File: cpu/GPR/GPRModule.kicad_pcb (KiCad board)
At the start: 2 copper layers, 100 x 80 mm, 52 parts, among them J1 Interconnect, U1 74HCT574, U10 74LHCT45, U11 74HCT125, U2 74HCT574, U3 74HCT245, U4 74HCT245, U5 74HCT245, U6 74HCT245, U7 74HCT245, U8 74HCT245, U9 74HCT245

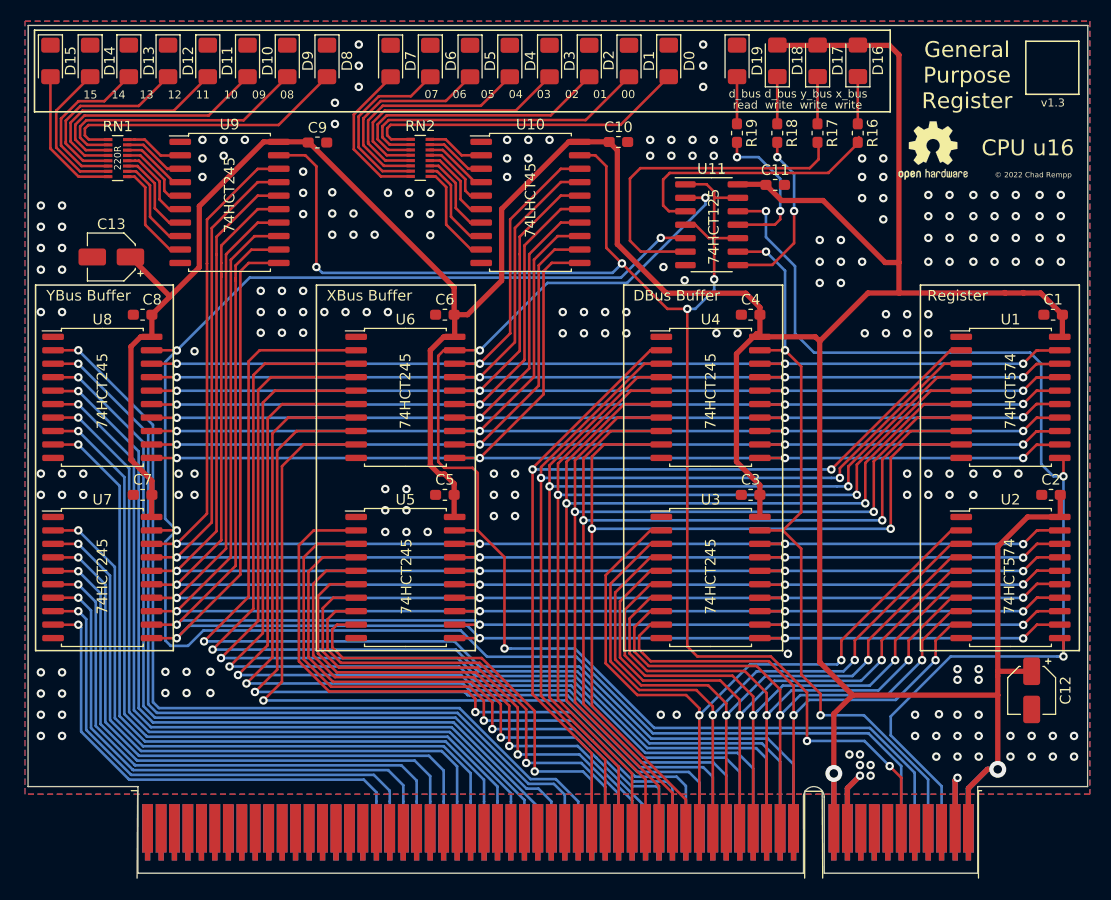
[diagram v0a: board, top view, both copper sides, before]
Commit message: Upgrade to KiCad 6 and commit a bunch of random stuff
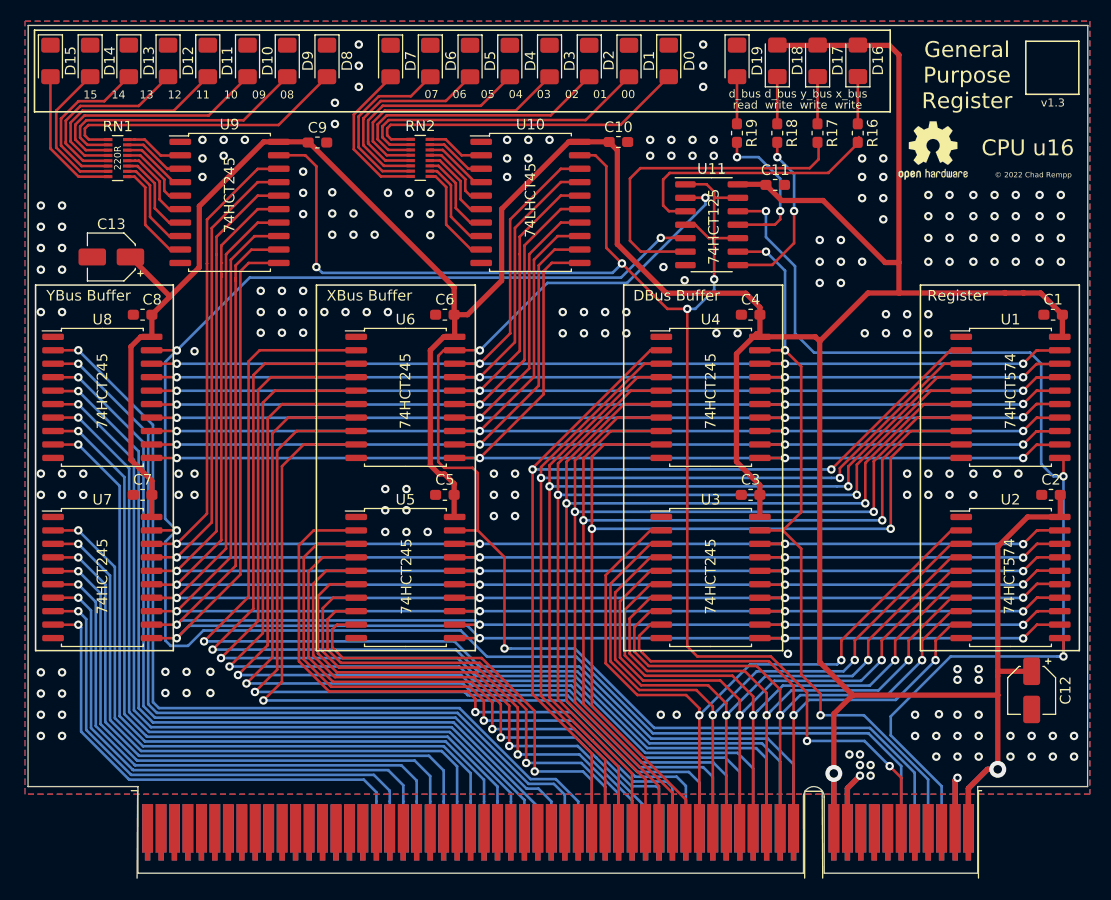
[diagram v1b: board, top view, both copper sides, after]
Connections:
- net /~DBG renamed /~{DBG}
- net /~d_bus_write renamed /~{d_bus_write}
- net /~x_bus_write renamed /~{x_bus_write}
- net /~y_bus_write renamed /~{y_bus_write}
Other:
- net class Default removed
- net class Power removed
